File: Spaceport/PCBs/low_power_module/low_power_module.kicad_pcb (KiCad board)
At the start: 2 copper layers, 37.5 x 32 mm, 39 parts, among them J1 SMA, U1 Si4463

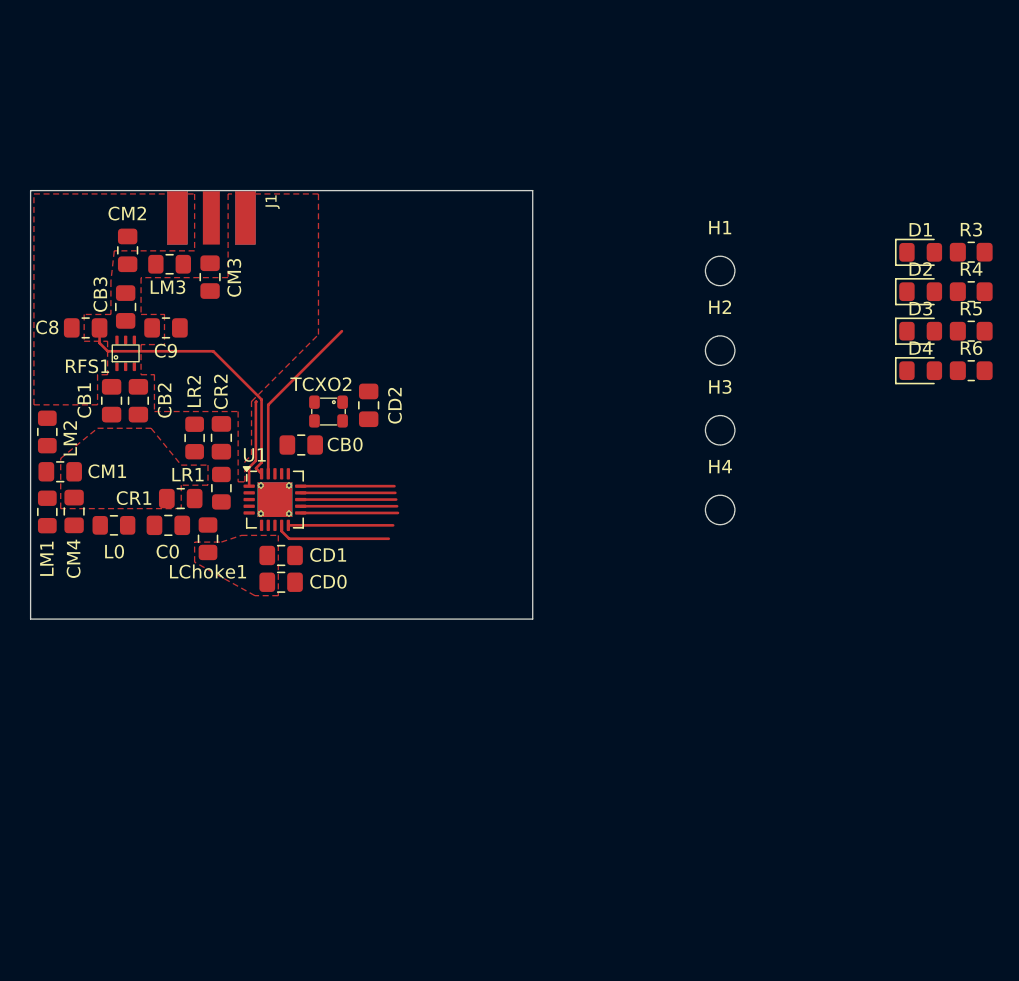
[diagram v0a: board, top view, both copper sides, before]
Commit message: Edited Trace Width on 50Ω microstrip and Changed Layout with New Filter
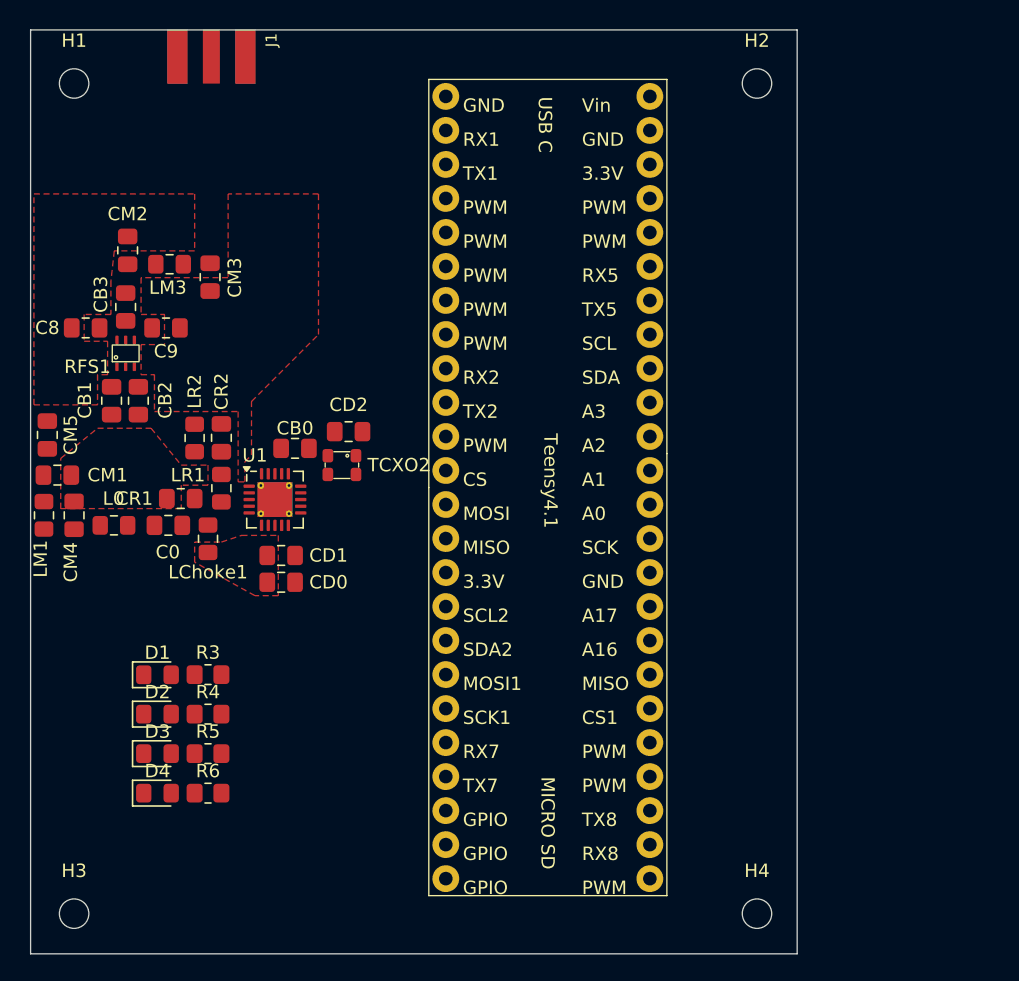
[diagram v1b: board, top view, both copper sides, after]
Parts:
- removed LM2: 56nH, Inductor_SMD:L_0805_2012Metric_Pad1.15x1.40mm_HandSolder
- added CM5: 22pF, Capacitor_SMD:C_0805_2012Metric_Pad1.18x1.45mm_HandSolder, F.Cu at (109.8, 96.0)
- added Teensy4.1: ~, SRAD_Avionics:Teensy_4.1, F.Cu at (147.1, 99.9)
- CM1: value 4.7pF -> 22pF
- LM1: value 56nH -> 10nH
- moved R3 65.1 mm to (121.8, 113.9)
- moved D1 65.1 mm to (118.0, 113.9)
- moved D2 65.1 mm to (118.0, 116.8)
- moved D3 65.1 mm to (118.0, 119.8)
- moved D4 65.1 mm to (118.0, 122.8)
- moved R4 65.1 mm to (121.8, 116.8)
- moved R5 65.1 mm to (121.8, 119.8)
- moved R6 65.1 mm to (121.8, 122.8)
- moved H3 60.3 mm to (111.8, 131.8)
- moved H1 50.2 mm to (111.8, 69.8)
- moved H4 30.3 mm to (162.8, 131.8)
- moved H2 20.1 mm to (162.8, 69.8)
- moved J1 12.0 mm to (122.0, 65.7)
- moved TCXO2 4.12 mm to (131.8, 98.2)
- moved CD2 2.47 mm to (132.2, 95.8), turned to 180 degrees
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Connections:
- CM4 pad 1: Net-(CM4-Pad1) -> Net-(CM1-Pad1)
- L0 pad 2: Net-(CM4-Pad1) -> Net-(CM1-Pad1)
- LM1 pad 1: Net-(CM4-Pad1) -> Net-(CM1-Pad1)
- LM1 pad 2: Net-(CM1-Pad1) -> RF2
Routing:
- net GPIO3: track 20.9 -> 0.00 mm
- net GPIO2: track 12.9 -> 0.00 mm
- net GPIO0: track 8.67 -> 0.00 mm
- net GPIO1: track 7.83 -> 0.00 mm
- net IRQ: track 7.26 -> 0.00 mm
- net SCLK: track 7.20 -> 0.00 mm
- net MISO: track 7.13 -> 0.00 mm
- net MOSI: track 7.07 -> 0.00 mm
- net CS: track 7.00 -> 0.00 mm
- net SDN: track 6.52 -> 0.00 mm
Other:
- board size 37.5 x 32 mm -> 57.2 x 69 mm
